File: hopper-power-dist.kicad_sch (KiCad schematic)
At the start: 29 parts, among them J1 XT60PW-M, J2 XT60PW-M, J3 B2B-XH-A(LF)(SN), J4 B2B-XH-A(LF)(SN), J5 XT60-F, J6 XT60PW-F, J7 XT60PW-F, J8 XT60PW-F, J9 XT60PW-F, SW1 FT_Power_Switch

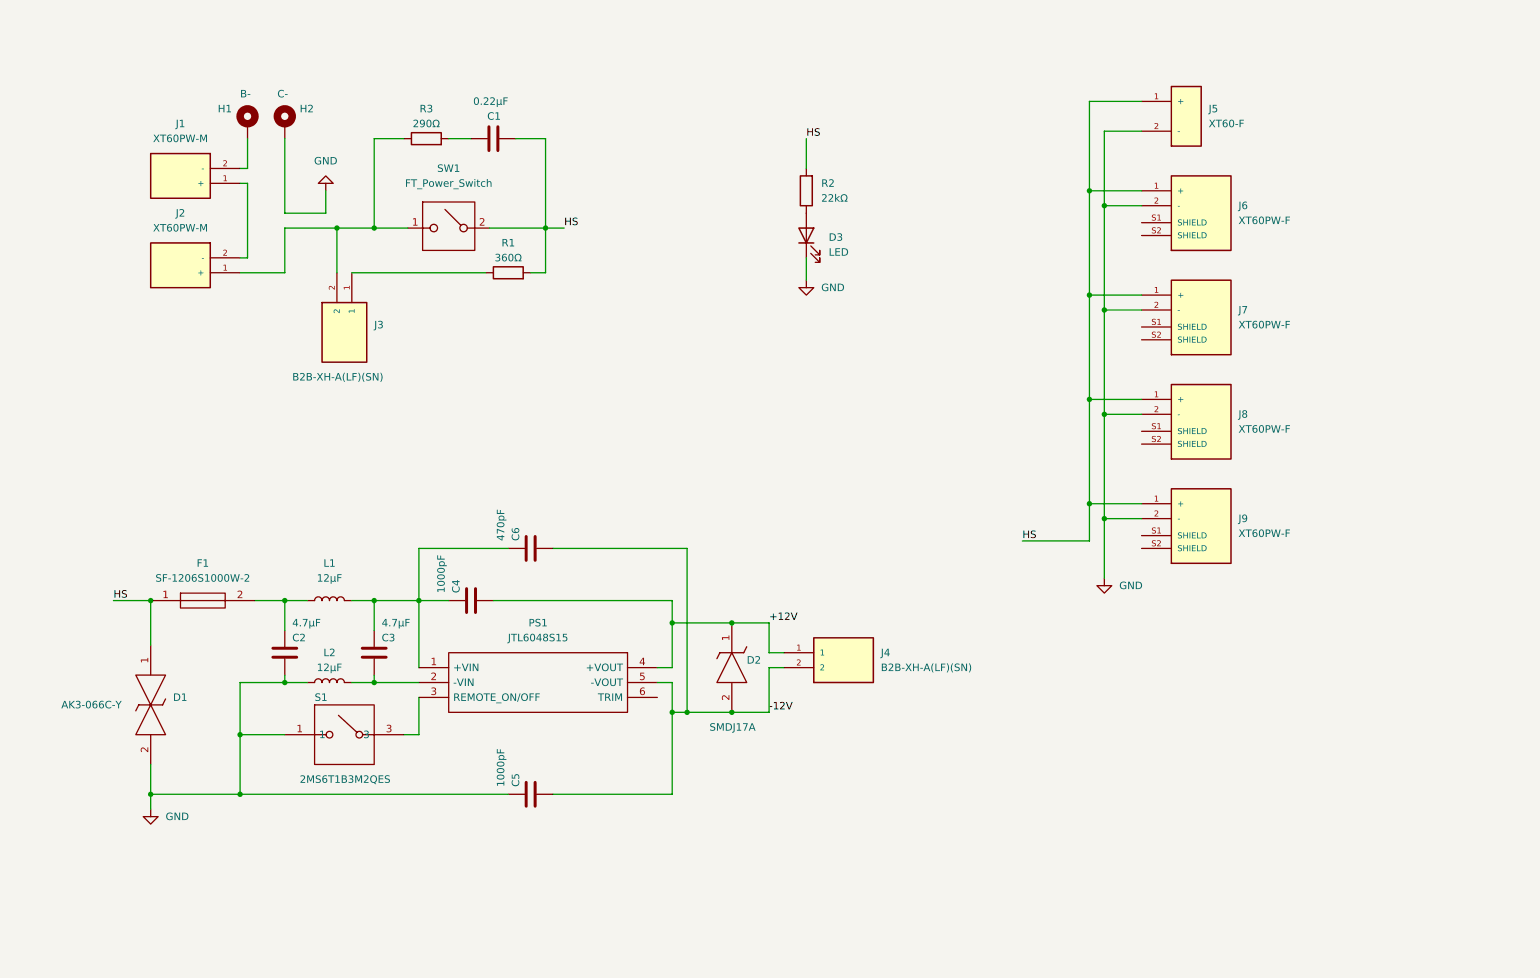
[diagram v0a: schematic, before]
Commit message: Started rev03 design
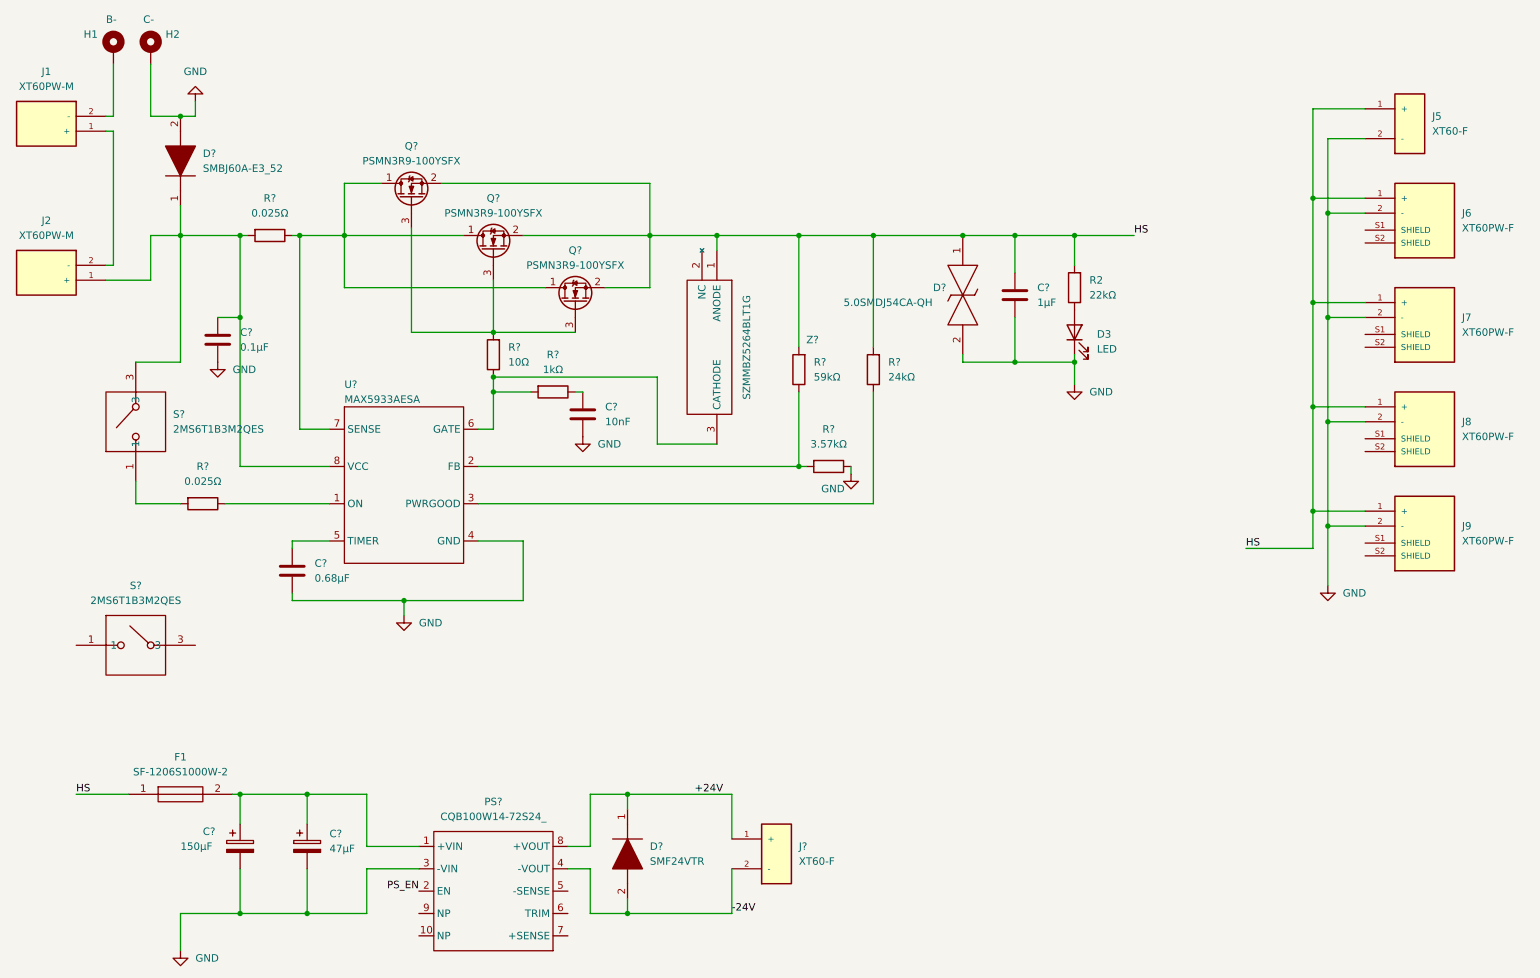
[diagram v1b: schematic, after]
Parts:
- removed C1: 0.22μF, Capacitor_SMD:C_1206_3216Metric, symbol Device:C
- removed C2: 4.7μF, SamacSys_Parts:CAPC3225X270N, symbol Device:C
- removed C3: 4.7μF, Capacitor_SMD:C_0805_2012Metric, symbol Device:C
- removed C4, C5: 1000pF, Capacitor_SMD:C_1206_3216Metric, symbol Device:C
- removed C6: 470pF, Capacitor_SMD:C_1206_3216Metric, symbol Device:C
- removed D1: AK3-066C-Y, SamacSys_Parts:AK3066CY, symbol AK3-066C-Y:AK3-066C-Y
- removed D2: SMDJ17A, DIOM7959X262N, symbol SamacSys_Parts:SMDJ17A
- removed J3, J4: B2B-XH-A(LF)(SN), JST_B2B-XH-A(LF)(SN), symbol B2B-XH-A_LF__SN_:B2B-XH-A(LF)(SN)
- removed L1, L2: 12μF, SamacSys_Parts:LPS6235123MRC, symbol Device:L
- removed PS1: JTL6048S15, JTL6048S15, symbol SamacSys_Parts:JTL6048S15
- removed R1: 360Ω, benbokser:AC03000003600JAC00, symbol Device:R
- removed R3: 290Ω, Resistor_SMD:R_2512_6332Metric, symbol Device:R
- removed S1: 2MS6T1B3M2QES, 2MS6T1B3M2QES, symbol benbokser:2MS6T1B3M2QES
- removed SW1: FT_Power_Switch, benbokser:FT Power Switch, symbol benbokser:FT_Power_Switch
- added C?: 10nF, symbol Device:C
- added C?: 1μF, symbol Device:C
- added C?: 150μF, symbol Device:C_Polarized
- added C?: 47μF, symbol Device:C_Polarized
- added C?: 0.68μF, symbol Device:C
- added C?: 0.1μF, symbol Device:C
- added D?: SMBJ60A-E3_52, DIOM5436X244N, symbol SamacSys_Parts:SMBJ60A-E3_52
- added D?: 5.0SMDJ54CA-QH, DIONM7959X262N, symbol SamacSys_Parts:5.0SMDJ54CA-QH
- added D?: SMF24VTR, SMF24VTR, symbol SamacSys_Parts:SMF24VTR
- added J?: XT60-F, XT60PW-F:AMASS_XT60-F, symbol XT60PW-F:XT60-F
- added PS?: CQB100W14-72S24_, symbol custom-symbols:CQB100W14-72S24_
- added Q? (x3): PSMN3R9-100YSFX, symbol custom-symbols:PSMN3R9-100YSFX
- added R?: 1kΩ, Resistor_SMD:R_0603_1608Metric_Pad0.98x0.95mm_HandSolder, symbol Device:R
- added R?: 59kΩ, Resistor_SMD:R_0603_1608Metric_Pad0.98x0.95mm_HandSolder, symbol Device:R
- added R?: 24kΩ, Resistor_SMD:R_0603_1608Metric_Pad0.98x0.95mm_HandSolder, symbol Device:R
- added R?: 10Ω, Resistor_SMD:R_0603_1608Metric_Pad0.98x0.95mm_HandSolder, symbol Device:R
- added R?: 3.57kΩ, Resistor_SMD:R_0603_1608Metric_Pad0.98x0.95mm_HandSolder, symbol Device:R
- added R? (x2): 0.025Ω, Resistor_SMD:R_0603_1608Metric_Pad0.98x0.95mm_HandSolder, symbol Device:R
- added S? (x2): 2MS6T1B3M2QES, 2MS6T1B3M2QES, symbol 2ms6t1b3m2qes:2MS6T1B3M2QES
- added U?: MAX5933AESA, symbol custom-symbols:MAX5933AESA
- added Z?: SZMMBZ5264BLT1G, SOT96P237X111-3N, symbol SamacSys_Parts:SZMMBZ5264BLT1G
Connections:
- net GND: now also C?.2, C?.2, C?.2, C?.2, C?.2, C?.2, D?.2, D?.2, PS?.3 (-VIN), R?.1, U?.4 (GND)
- net HS: now also C?.1, D?.1, Q?.2 (S), Q?.2 (S), Q?.2 (S), R?.2, R?.2, Z?.1 (ANODE)
- net at J2.1 (+): now also C?.1, D?.1, R?.2, S?.3, U?.8 (VCC)
- net at F1.2: now also C?.1, C?.1, PS?.1 (+VIN)
- new net: C?.1, R?.1
- new net: R?.1, R?.2, U?.6 (GATE), Z?.3 (CATHODE)
- new net: R?.2, S?.1
- new net: Q?.1 (D), Q?.1 (D), Q?.1 (D), R?.1, U?.7 (SENSE)
- new net: Q?.3 (G), Q?.3 (G), Q?.3 (G), R?.2
- new net: R?.1, R?.2, U?.2 (FB)
- new net: R?.1, U?.1 (ON)
- new net: R?.1, U?.3 (PWRGOOD)
- new net: C?.1, U?.5 (TIMER)
- new net +24V: D?.1, J?.1 (+), PS?.8 (+VOUT)
- new net -24V: D?.2, J?.2 (-), PS?.4 (-VOUT)
- new net PS_EN: PS?.2 (EN)
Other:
- moved on the sheet: D3, F1, H1, H2, J1, J2, J5, J6, J7, J8, J9, R2
